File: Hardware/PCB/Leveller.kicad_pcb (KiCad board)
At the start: 2 copper layers, 20 x 27.8 mm, 32 parts, among them J12 Conn_01x06_Socket, J7 Conn_01x05_Pin, U1 TL074, U2 TL074

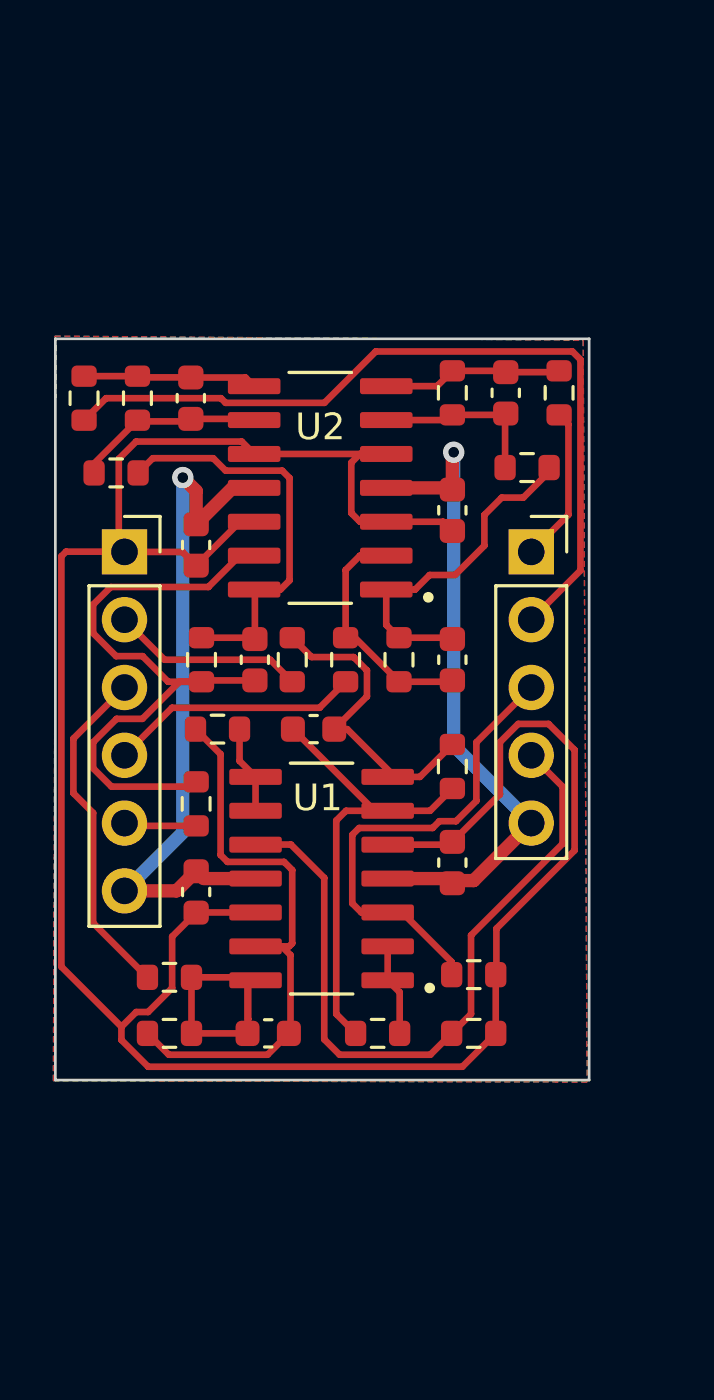
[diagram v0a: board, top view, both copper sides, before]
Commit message: Version 1.0 of hardware ordered
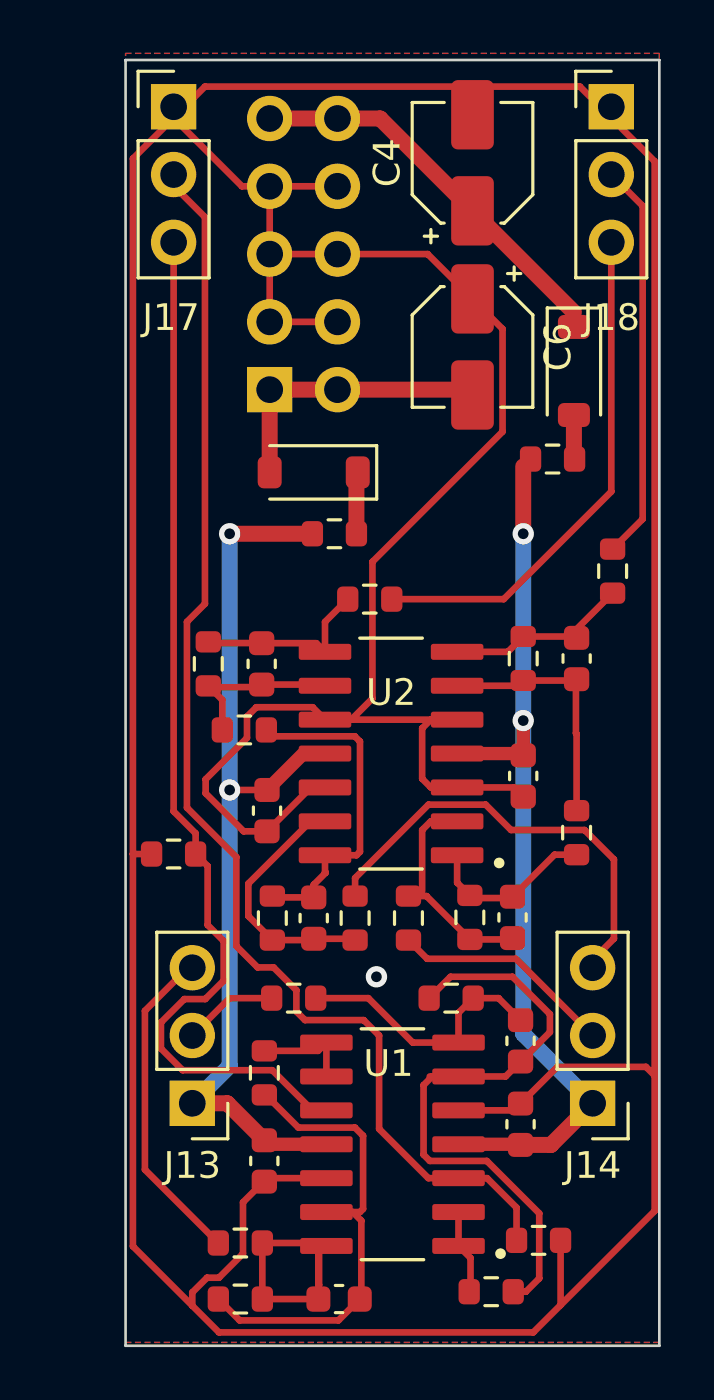
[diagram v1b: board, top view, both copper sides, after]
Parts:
- removed J12: Conn_01x06_Socket, Connector_PinSocket_2.54mm:PinSocket_1x06_P2.54mm_Vertical
- removed J7: Conn_01x05_Pin, Connector_PinSocket_2.54mm:PinSocket_1x05_P2.54mm_Vertical
- added C4: 10uF, Capacitor_SMD:CP_Elec_4x5.4, F.Cu at (63.0, 44.2)
- added C6: 10uF, Capacitor_SMD:CP_Elec_4x5.4, F.Cu at (63.0, 51.1)
- added D1: 1N5819, Diode_SMD:D_SOD-123, F.Cu at (57.0, 55.8)
- added D4: 1N5819, Diode_SMD:D_SOD-123, F.Cu at (66.8, 52.0)
- added FB1: FerriteBead, Resistor_SMD:R_0603_1608Metric, F.Cu at (57.8, 58.1)
- added FB2: FerriteBead, Resistor_SMD:R_0603_1608Metric, F.Cu at (66.0, 55.3)
- added J13: Audio to Daisy, connect to J13, Connector_PinHeader_2.54mm:PinHeader_1x03_P2.54mm_Vertical, F.Cu at (52.5, 79.4)
- added J14: Audio from Daisy, connect to J10, Connector_PinHeader_2.54mm:PinHeader_1x03_P2.54mm_Vertical, F.Cu at (67.5, 79.4)
- added J17: Audio output, connect to J16, Connector_PinHeader_2.54mm:PinHeader_1x03_P2.54mm_Vertical, F.Cu at (51.8, 42.1)
- added J18: Audio input, connect to J15, Connector_PinHeader_2.54mm:PinHeader_1x03_P2.54mm_Vertical, F.Cu at (68.2, 42.1)
- added J6: Eurorack_Power, Connector_PinHeader_2.54mm:PinHeader_2x05_P2.54mm_Vertical, B.Cu at (55.4, 52.7)
- moved C2 14.0 mm to (64.8, 77.1), turned to 90 degrees
- moved R15 13.8 mm to (66.9, 69.3), turned to -90 degrees
- moved R9 13.1 mm to (51.8, 70.1), turned to 180 degrees
- moved R22 13.1 mm to (59.1, 60.5), turned to 180 degrees
- moved R10 13.0 mm to (55.2, 78.3), turned to -90 degrees
- moved R8 12.7 mm to (56.3, 75.5), turned to 180 degrees
- moved R20 10.8 mm to (54.5, 65.5)
- moved R6 10.6 mm to (63.7, 86.5), turned to 0 degrees
- moved C5 10.4 mm to (55.2, 81.6)
- moved C3 10.3 mm to (58.0, 86.8)
- moved R11 10.3 mm to (54.3, 86.8)
- moved C12 10.3 mm to (64.9, 67.2)
- moved R17 10.3 mm to (64.9, 62.8)
- moved C8 10.3 mm to (66.9, 62.8)
- moved C9 10.3 mm to (55.1, 63.0)
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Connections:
- R12 pad 2: Net-(J12-Pin_3) -> (no net)
- R14 pad 2: Net-(J12-Pin_4) -> (no net)
- R16 pad 1: Net-(J7-Pin_1) -> (no net)
- R21 pad 2: Net-(J12-Pin_5) -> (no net)
- R22 pad 1: Net-(J7-Pin_2) -> (no net)
- R5 pad 1: Net-(J7-Pin_3) -> (no net)
- R8 pad 2: Net-(J12-Pin_2) -> (no net)
- R9 pad 1: Net-(J7-Pin_4) -> (no net)
- U1 pad 10: Net-(J7-Pin_4) -> (no net)
- U1 pad 3: Net-(J7-Pin_3) -> (no net)
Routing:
- net (no net): track 0.00 -> 190.9 mm
- net GND: track 92.8 -> 211.1 mm, vias 0 -> 1
- net Net-(J7-Pin_2): track 30.4 -> 0.00 mm
- net Net-(J7-Pin_4): track 27.1 -> 0.00 mm
- net Net-(J7-Pin_3): track 17.4 -> 0.00 mm
- net Net-(U2D--): track 24.0 -> 8.79 mm
- net Net-(J12-Pin_3): track 12.8 -> 0.00 mm
- net +12V: track 25.0 -> 34.9 mm, vias 1 -> 2
- net Net-(J12-Pin_4): track 9.43 -> 0.00 mm
- net -12V: track 25.2 -> 33.6 mm, vias 1 -> 2
- net Net-(J12-Pin_2): track 7.25 -> 0.00 mm
- net Net-(U1B--): track 17.4 -> 24.2 mm
- net Net-(C7-Pad2): track 12.6 -> 6.55 mm
- net Net-(J7-Pin_1): track 5.86 -> 0.00 mm
- net Net-(U1D--): track 22.5 -> 18.7 mm
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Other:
- board size 20 x 27.8 mm -> 20 x 48.2 mm
- board text added: "Loop v1.0"
- board text added: "Serial"
- board text added: "by Geir & Adam"
- board text added: "https://github.com/GugeNet/Loop"
